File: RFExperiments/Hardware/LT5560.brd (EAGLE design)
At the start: 50 x 50 mm, 47 parts, among them IC1 LT5560, IC2 LTC6362, IC3 VREG-TS1117CW-5V, Q1 BSS123, Q2 BSS123, X1 IN, X2 LO

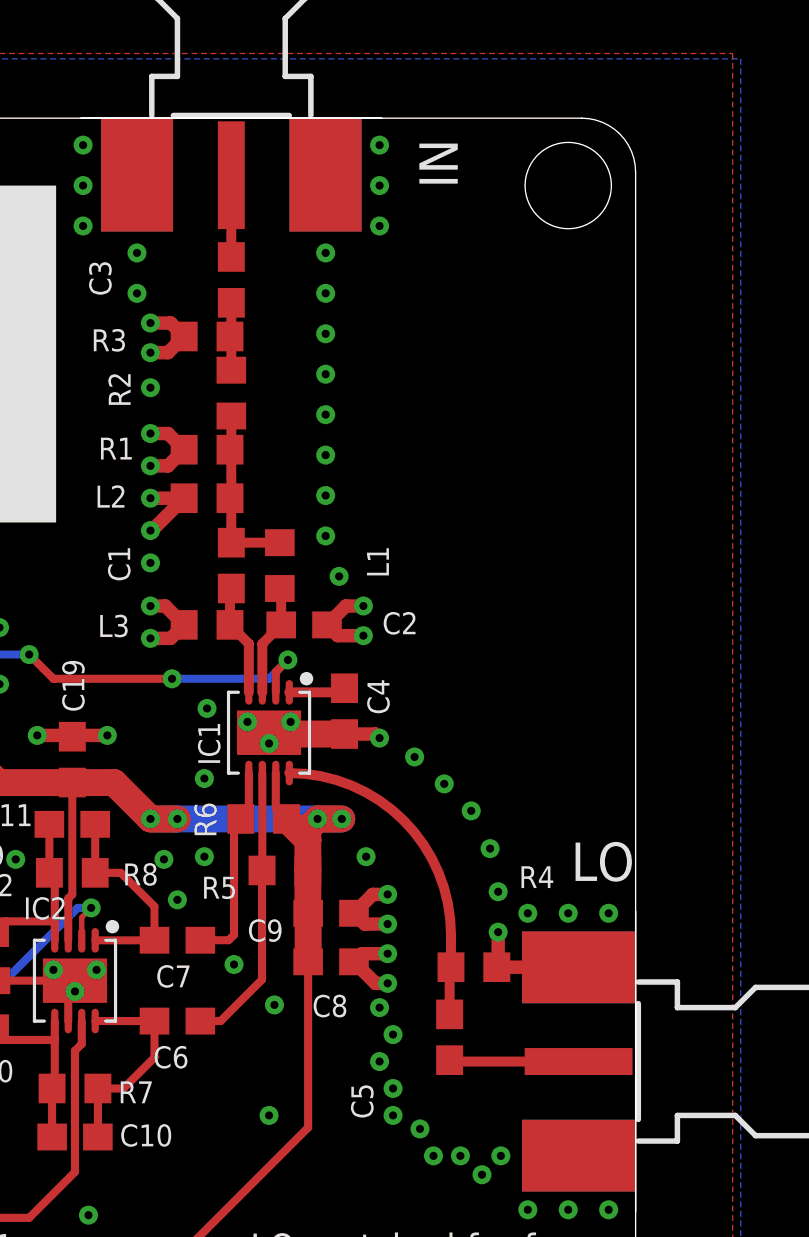
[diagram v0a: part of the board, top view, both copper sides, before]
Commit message: Gerber and BOM
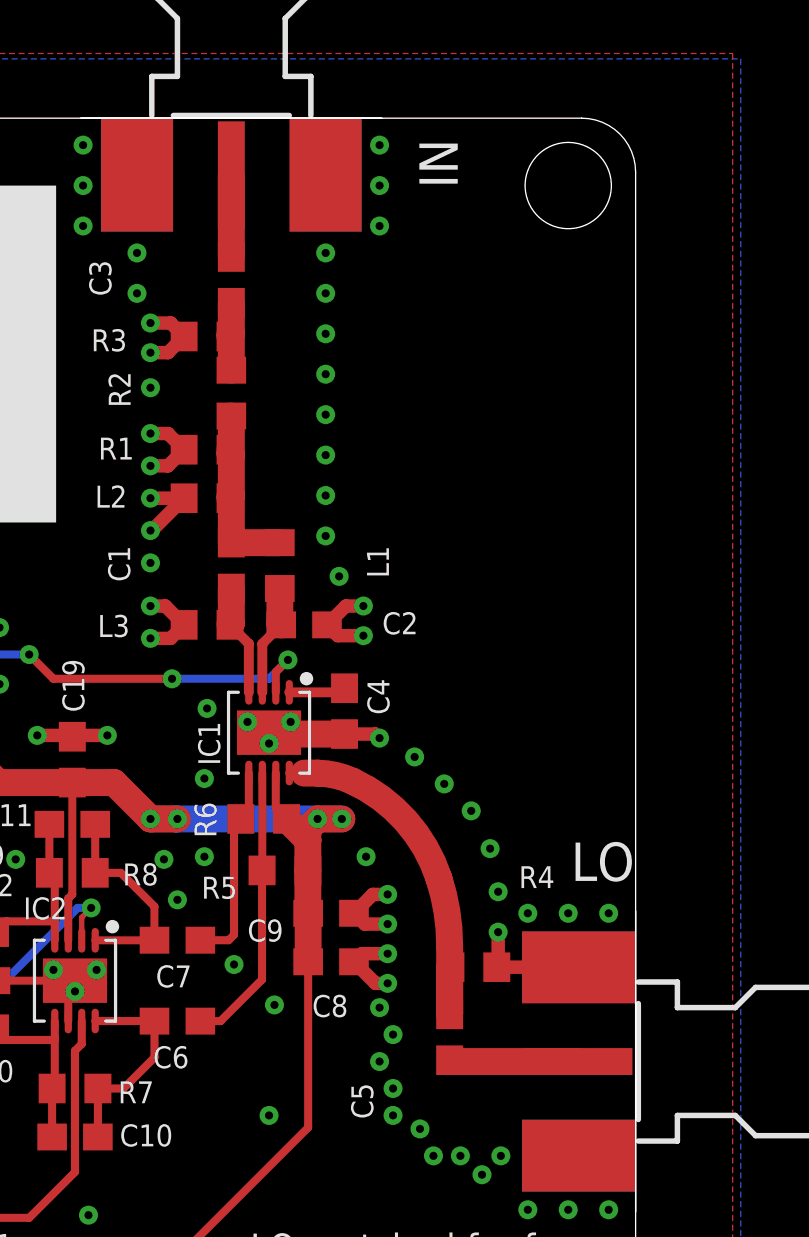
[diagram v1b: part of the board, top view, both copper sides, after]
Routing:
- net N$7: track 11.5 -> 14.1 mm
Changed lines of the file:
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@@
 <layers>
 <layer number="1" name="Top" color="4" fill="1" visible="yes" active="yes"/>
-<layer number="2" name="Route2" color="10" fill="1" visible="no" active="yes"/>
+<layer number="2" name="Route2" color="10" fill="1" visible="no" active="no"/>
 <layer number="3" name="Route3" color="17" fill="1" visible="no" active="no"/>
 <layer number="4" name="Route4" color="18" fill="1" visible="no" active="no"/>
@@
 <layer number="13" name="Route13" color="21" fill="1" visible="no" active="no"/>
 <layer number="14" name="Route14" color="22" fill="1" visible="no" active="no"/>
-<layer number="15" name="Route15" color="14" fill="1" visible="no" active="yes"/>
+<layer number="15" name="Route15" color="14" fill="1" visible="no" active="no"/>
 <layer number="16" name="Bottom" color="1" fill="1" visible="yes" active="yes"/>
 <layer number="17" name="Pads" color="2" fill="1" visible="yes" active="yes"/>
@@
 </class>
 </classes>
-<designrules name="JLCPCB4L_7628">
+<designrules name="JLCPCB4L_7628 *">
 <description language="de">&lt;b&gt;EAGLE Design Rules&lt;/b&gt;
 &lt;p&gt;
@@
 necessary adjustments and save your customized
 design rules under a new name.</description>
-<param name="layerSetup" value="(1+2*15+16)"/>
+<param name="layerSetup" value="(1*16)"/>
 <param name="mtCopper" value="0.035mm 0.0175mm 0.035mm 0.035mm 0.035mm 0.035mm 0.035mm 0.035mm 0.035mm 0.035mm 0.035mm 0.035mm 0.035mm 0.035mm 0.0175mm 0.035mm"/>
 <param name="mtIsolate" value="0.2mm 1.064mm 0.2mm 0.15mm 0.2mm 0.15mm 0.2mm 0.15mm 0.2mm 0.15mm 0.2mm 0.15mm 0.2mm 0.15mm 0.2mm"/>
@@
 <wire x1="35.65" y1="28.6973" x2="35.65" y2="30.5" width="0.37" layer="1"/>
 <wire x1="35.65" y1="30.5" x2="34.95" y2="31.2" width="0.37" layer="1"/>
-<wire x1="34.95" y1="31.2" x2="34.95" y2="32.5" width="0.37" layer="1"/>
 <wire x1="34.95" y1="32.5" x2="35" y2="32.55" width="0.37" layer="1"/>
+<wire x1="35" y1="32.55" x2="35" y2="31.25" width="1" layer="1"/>
+<wire x1="35" y1="31.25" x2="34.95" y2="31.2" width="1" layer="1"/>
 </signal>
 <signal name="N$2">
@@
 <wire x1="36.15" y1="28.6973" x2="36.15" y2="30.5" width="0.37" layer="1"/>
 <wire x1="36.15" y1="30.5" x2="36.85" y2="31.2" width="0.37" layer="1"/>
-<wire x1="36.85" y1="31.2" x2="36.85" y2="32.5" width="0.37" layer="1"/>
 <wire x1="36.85" y1="32.5" x2="36.8" y2="32.55" width="0.37" layer="1"/>
+<wire x1="36.8" y1="32.55" x2="36.8" y2="31.25" width="1" layer="1"/>
+<wire x1="36.8" y1="31.25" x2="36.85" y2="31.2" width="1" layer="1"/>
 </signal>
 <signal name="N$3">
@@
 <contactref element="R2" pad="1"/>
 <contactref element="R1" pad="2"/>
-<wire x1="35" y1="34.25" x2="35" y2="35.9" width="0.37" layer="1"/>
-<wire x1="35" y1="35.9" x2="35" y2="37.7" width="0.37" layer="1"/>
-<wire x1="35" y1="37.7" x2="35" y2="38.95" width="0.37" layer="1"/>
 <wire x1="34.95" y1="37.7" x2="35" y2="37.7" width="0.37" layer="1"/>
 <wire x1="34.95" y1="35.9" x2="35" y2="35.9" width="0.37" layer="1"/>
-<wire x1="35" y1="34.25" x2="36.8" y2="34.25" width="0.37" layer="1"/>
+<wire x1="35" y1="38.95" x2="35" y2="37.5" width="1" layer="1"/>
+<wire x1="35" y1="37.5" x2="35" y2="36" width="1" layer="1"/>
+<wire x1="35" y1="36" x2="35" y2="34.25" width="1" layer="1"/>
+<wire x1="34.95" y1="35.9" x2="34.95" y2="35.95" width="1" layer="1"/>
+<wire x1="34.95" y1="35.95" x2="35" y2="36" width="1" layer="1"/>
+<wire x1="34.95" y1="37.7" x2="34.95" y2="37.55" width="1" layer="1"/>
+<wire x1="34.95" y1="37.55" x2="35" y2="37.5" width="1" layer="1"/>
+<wire x1="35" y1="34.25" x2="36.8" y2="34.25" width="1" layer="1"/>
 </signal>
 <signal name="N$4">
 <contactref element="X1" pad="1"/>
 <contactref element="C3" pad="1"/>
-<wire x1="35" y1="47.8846" x2="35" y2="44.85" width="0.37" layer="1"/>
+<wire x1="35" y1="44.85" x2="35" y2="47.8846" width="1" layer="1"/>
 </signal>
 <signal name="N$5">
@@
 <contactref element="R2" pad="2"/>
 <contactref element="R3" pad="1"/>
-<wire x1="35" y1="40.65" x2="35" y2="41.9" width="0.37" layer="1"/>
-<wire x1="35" y1="41.9" x2="35" y2="43.15" width="0.37" layer="1"/>
 <wire x1="34.95" y1="41.9" x2="35" y2="41.9" width="0.37" layer="1"/>
+<wire x1="35" y1="43.15" x2="35" y2="42" width="1" layer="1"/>
+<wire x1="35" y1="42" x2="35" y2="40.65" width="1" layer="1"/>
+<wire x1="34.95" y1="41.9" x2="34.95" y2="41.95" width="1" layer="1"/>
+<wire x1="34.95" y1="41.95" x2="35" y2="42" width="1" layer="1"/>
 </signal>
 <signal name="N$6">
@@
 <contactref element="C5" pad="2"/>
 <contactref element="R4" pad="1"/>
-<wire x1="43.1" y1="16.75" x2="43.1" y2="18.45" width="0.37" layer="1"/>
 <wire x1="43.1" y1="18.45" x2="43.15" y2="18.5" width="0.37" layer="1"/>
-<wire x1="43.15" y1="18.5" x2="43.15" y2="19.7027" width="0.37" layer="1"/>
-<wire x1="43.15" y1="19.7027" x2="37.15" y2="25.7027" width="0.37" layer="1" curve="90"/>
+<wire x1="43.1" y1="16.75" x2="43.1" y2="18.45" width="1" layer="1"/>
+<wire x1="43.1" y1="16.75" x2="43.1" y2="19.3" width="1" layer="1"/>
+<wire x1="43.1" y1="19.3" x2="42.7" y2="21.8" width="1" layer="1" curve="18.180554"/>
+<wire x1="42.7" y1="21.8" x2="39.5" y2="25.4" width="1" layer="1" curve="46.90599"/>
+<wire x1="39.5" y1="25.4" x2="38.2" y2="25.7" width="1" layer="1" curve="23.83765"/>
+<wire x1="38.2" y1="25.7" x2="37.7" y2="25.7" width="1" layer="1" curve="2.151475"/>
+<wire x1="37.7" y1="25.7" x2="37.15" y2="25.7027" width="0.3048" layer="1" curve="-2.714011"/>
 </signal>
 <signal name="N$8">
 <contactref element="C5" pad="1"/>
 <contactref element="X2" pad="1"/>
-<wire x1="47.8846" y1="15" x2="43.15" y2="15" width="0.37" layer="1"/>
 <wire x1="43.15" y1="15" x2="43.1" y2="15.05" width="0.37" layer="1"/>
+<wire x1="47.8846" y1="15" x2="43.15" y2="15" width="1" layer="1"/>
 </signal>
 <signal name="N$10">

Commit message: Bugfixes and tests
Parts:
- C12: value DNP -> 100n
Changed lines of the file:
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@@
 <attribute name="VALUE" x="28.465" y="21.895" size="1.27" layer="27"/>
 </element>
-<element name="C12" library="resistor" package="C0603" value="DNP" x="25.4" y="18" smashed="yes">
+<element name="C12" library="resistor" package="C0603" value="100n" x="25.4" y="18" smashed="yes">
 <attribute name="NAME" x="24.965" y="21.135" size="0.8128" layer="25" font="vector"/>
 <attribute name="VALUE" x="24.765" y="16.095" size="1.27" layer="27"/>
